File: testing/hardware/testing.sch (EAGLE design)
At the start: 17 parts, among them J1 SPI_COMM, X1 POWER, X2 CAN_HI_LO

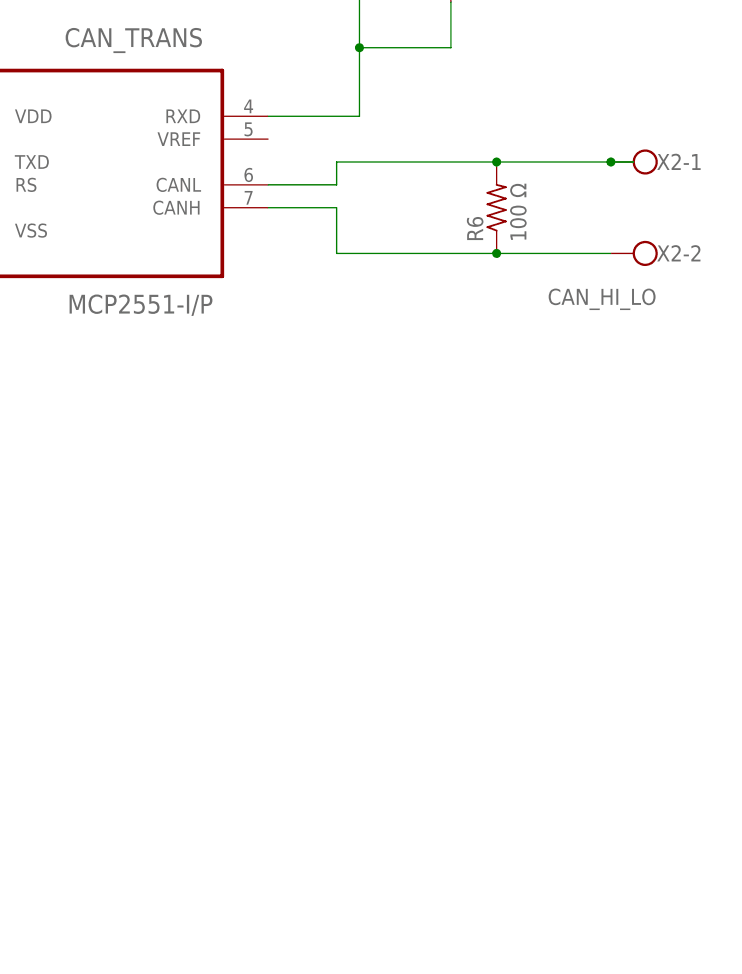
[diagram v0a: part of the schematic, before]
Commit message: test module updates
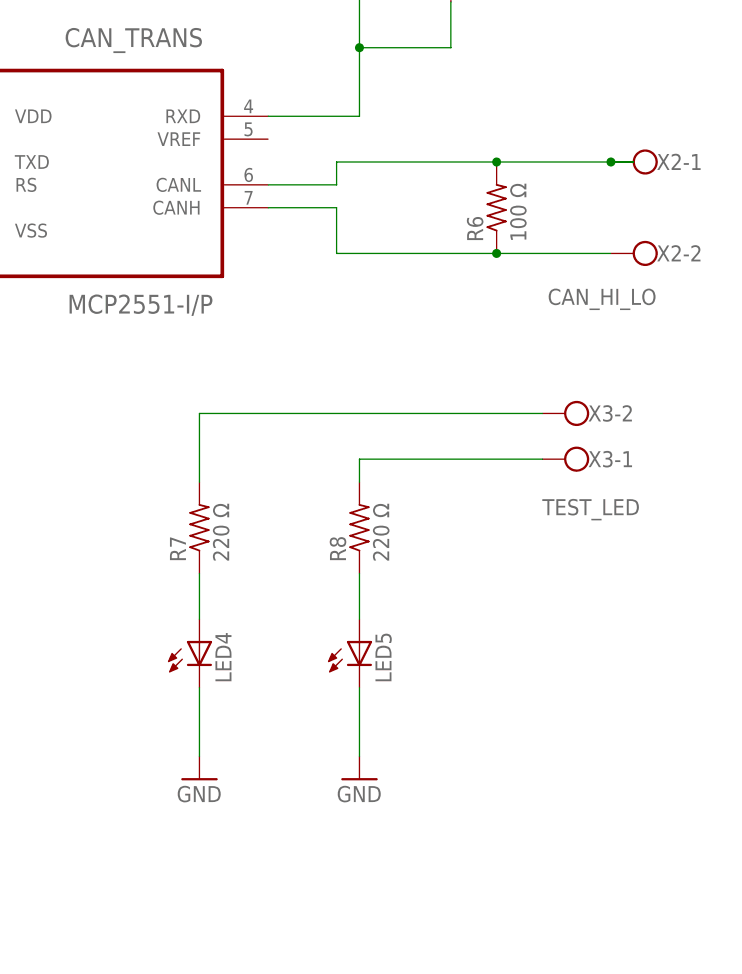
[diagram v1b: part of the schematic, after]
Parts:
- added LED4, LED5: (no value), adafruit:LED5MM
- added R7, R8: 220 Ω, adafruit:R-US_0204/7
- added X3: TEST_LED, con-wago-500:W237-102
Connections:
- net N$1 renamed RXCAN
- net N$10 renamed CS
- net N$11 renamed SCK
- net N$12 renamed CAN_H
- net N$14 renamed SI
- net N$15 renamed SO
- net N$17 renamed CAN_L
- net N$2 renamed TXCAN
- net N$7 renamed INT
- new net N$1: R7.2, X3-2.KL
- new net N$10: LED5.A, R8.1
- new net N$2: R8.2, X3-1.KL
- new net N$7: LED4.A, R7.1
- net GND: now also LED4.C, LED5.C
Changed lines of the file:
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@@
 <part name="J1" library="con-amp" deviceset="MTA05-156" device="" value="SPI_COMM"/>
 <part name="FRAME1" library="frames" library_urn="urn:adsk.eagle:library:229" deviceset="FRAME_A_L" device="" value="frame"/>
+<part name="LED4" library="adafruit" deviceset="LED" device="5MM"/>
+<part name="R7" library="adafruit" deviceset="R-US_" device="0204/7" value="220 Ω"/>
+<part name="LED5" library="adafruit" deviceset="LED" device="5MM"/>
+<part name="R8" library="adafruit" deviceset="R-US_" device="0204/7" value="220 Ω"/>
+<part name="GND5" library="SparkFun" deviceset="GND" device=""/>
+<part name="GND6" library="SparkFun" deviceset="GND" device=""/>
+<part name="X3" library="con-wago-500" deviceset="W237-102" device="" value="TEST_LED"/>
 </parts>
 <sheets>
@@
 <attribute name="DRAWING_NAME" x="185.42" y="19.05" size="2.54" layer="94"/>
 </instance>
+<instance part="LED4" gate="G$1" x="203.2" y="78.74" smashed="yes">
+<attribute name="NAME" x="206.756" y="74.168" size="1.778" layer="95" rot="R90"/>
+<attribute name="VALUE" x="208.915" y="74.168" size="1.778" layer="96" rot="R90"/>
+</instance>
+<instance part="R7" gate="G$1" x="203.2" y="91.44" smashed="yes" rot="R90">
+<attribute name="NAME" x="201.7014" y="87.63" size="1.778" layer="95" rot="R90"/>
+<attribute name="VALUE" x="206.502" y="87.63" size="1.778" layer="96" rot="R90"/>
+</instance>
+<instance part="LED5" gate="G$1" x="220.98" y="78.74" smashed="yes">
+<attribute name="NAME" x="224.536" y="74.168" size="1.778" layer="95" rot="R90"/>
+<attribute name="VALUE" x="226.695" y="74.168" size="1.778" layer="96" rot="R90"/>
+</instance>
+<instance part="R8" gate="G$1" x="220.98" y="91.44" smashed="yes" rot="R90">
+<attribute name="NAME" x="219.4814" y="87.63" size="1.778" layer="95" rot="R90"/>
+<attribute name="VALUE" x="224.282" y="87.63" size="1.778" layer="96" rot="R90"/>
+</instance>
+<instance part="GND5" gate="1" x="203.2" y="63.5" smashed="yes">
+<attribute name="VALUE" x="200.66" y="60.96" size="1.778" layer="96"/>
+</instance>
+<instance part="GND6" gate="1" x="220.98" y="63.5" smashed="yes">
+<attribute name="VALUE" x="218.44" y="60.96" size="1.778" layer="96"/>
+</instance>
+<instance part="X3" gate="-1" x="246.38" y="99.06" smashed="yes" rot="R180">
+<attribute name="NAME" x="246.38" y="98.171" size="1.778" layer="95"/>
+</instance>
+<instance part="X3" gate="-2" x="246.38" y="104.14" smashed="yes" rot="R180">
+<attribute name="VALUE" x="241.3" y="92.837" size="1.778" layer="96"/>
+<attribute name="NAME" x="246.38" y="103.251" size="1.778" layer="95"/>
+</instance>
 </instances>
 <busses>
 </busses>
 <nets>
-<net name="N$2" class="0">
+<net name="TXCAN" class="0">
 <segment>
 <pinref part="CAN_CONTRL" gate="A" pin="TXCAN"/>
@@
 </segment>
 </net>
-<net name="N$1" class="0">
+<net name="RXCAN" class="0">
 <segment>
 <pinref part="CAN_CONTRL" gate="A" pin="RXCAN"/>
@@
 <wire x1="162.56" y1="144.78" x2="157.48" y2="144.78" width="0.1524" layer="91"/>
 <wire x1="157.48" y1="144.78" x2="157.48" y2="139.7" width="0.1524" layer="91"/>
+</segment>
+<segment>
+<pinref part="LED4" gate="G$1" pin="C"/>
+<wire x1="203.2" y1="73.66" x2="203.2" y2="66.04" width="0.1524" layer="91"/>
+<pinref part="GND5" gate="1" pin="GND"/>
+</segment>
+<segment>
+<pinref part="LED5" gate="G$1" pin="C"/>
+<wire x1="220.98" y1="73.66" x2="220.98" y2="66.04" width="0.1524" layer="91"/>
+<pinref part="GND6" gate="1" pin="GND"/>
 </segment>
 </net>
@@
 </segment>
 </net>
-<net name="N$7" class="0">
+<net name="INT" class="0">
 <segment>
 <pinref part="LED1" gate="G$1" pin="C"/>
@@
 </segment>
 </net>
-<net name="N$12" class="0">
+<net name="CAN_H" class="0">
 <segment>
 <pinref part="CAN_TRANS" gate="A" pin="CANH"/>
@@
 </segment>
 </net>
-<net name="N$17" class="0">
+<net name="CAN_L" class="0">
 <segment>
 <wire x1="251.46" y1="132.08" x2="248.92" y2="132.08" width="0.1524" layer="91"/>
@@
 <junction x="248.92" y="132.08"/>
 <junction x="236.22" y="132.08"/>
-</segment>
-</net>
-<net name="N$11" class="0">
+<wire x1="251.46" y1="132.08" x2="248.92" y2="132.08" width="0.1524" layer="91"/>
+</segment>
+</net>
+<net name="SCK" class="0">
 <segment>
 <pinref part="CAN_CONTRL" gate="A" pin="SCK"/>
@@
 </segment>
 </net>
-<net name="N$14" class="0">
+<net name="SI" class="0">
 <segment>
 <pinref part="J1" gate="G$1" pin="2"/>
@@
 </segment>
 </net>
-<net name="N$15" class="0">
+<net name="SO" class="0">
 <segment>
 <pinref part="J1" gate="G$1" pin="3"/>
@@
 </segment>
 </net>
-<net name="N$10" class="0">
+<net name="CS" class="0">
 <segment>
 <pinref part="CAN_CONTRL" gate="A" pin="~CS"/>
@@
 </segment>
 </net>
+<net name="N$1" class="0">
+<segment>
+<pinref part="R7" gate="G$1" pin="2"/>
+<wire x1="203.2" y1="96.52" x2="203.2" y2="104.14" width="0.1524" layer="91"/>
+<wire x1="203.2" y1="104.14" x2="241.3" y2="104.14" width="0.1524" layer="91"/>
+<pinref part="X3" gate="-2" pin="KL"/>
+</segment>
+</net>
+<net name="N$2" class="0">
+<segment>
+<pinref part="R8" gate="G$1" pin="2"/>
+<wire x1="220.98" y1="96.52" x2="220.98" y2="99.06" width="0.1524" layer="91"/>
+<wire x1="220.98" y1="99.06" x2="241.3" y2="99.06" width="0.1524" layer="91"/>
+<pinref part="X3" gate="-1" pin="KL"/>
+</segment>
+</net>
+<net name="N$7" class="0">
+<segment>
+<pinref part="R7" gate="G$1" pin="1"/>
+<pinref part="LED4" gate="G$1" pin="A"/>
+<wire x1="203.2" y1="86.36" x2="203.2" y2="81.28" width="0.1524" layer="91"/>
+</segment>
+</net>
+<net name="N$10" class="0">
+<segment>
+<pinref part="R8" gate="G$1" pin="1"/>
+<pinref part="LED5" gate="G$1" pin="A"/>
+<wire x1="220.98" y1="86.36" x2="220.98" y2="81.28" width="0.1524" layer="91"/>
+</segment>
+</net>
